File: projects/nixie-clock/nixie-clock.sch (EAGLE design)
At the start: 75 parts, among them J1 POWER JACK, T1 BC337, T2 BC337, T3 BC337, U1 DC-DC Converter, U2 K155ID1, U3 Arduino Pro Mini, U4 Pollin DCF1, U5 REG1117

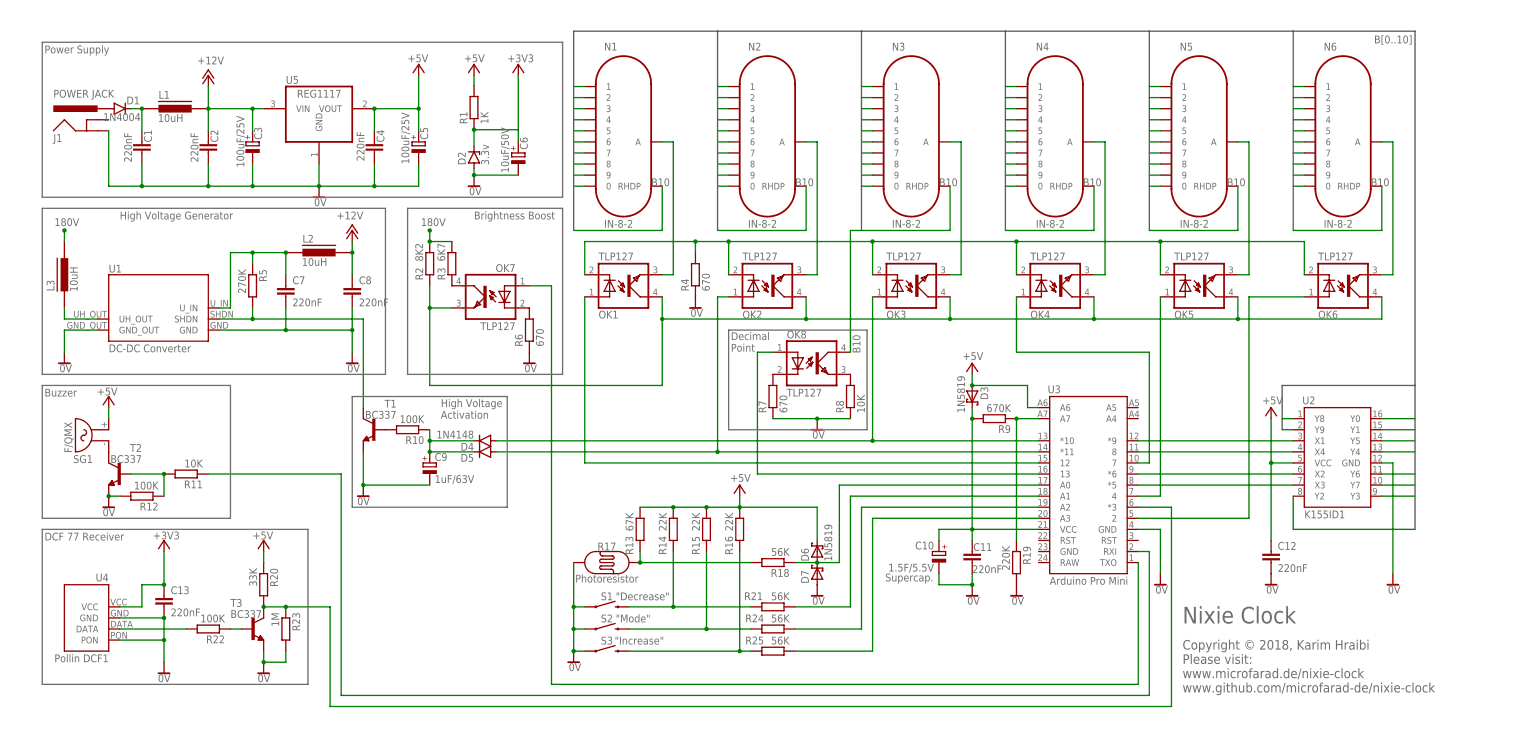
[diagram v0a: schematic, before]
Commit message: Update schematic
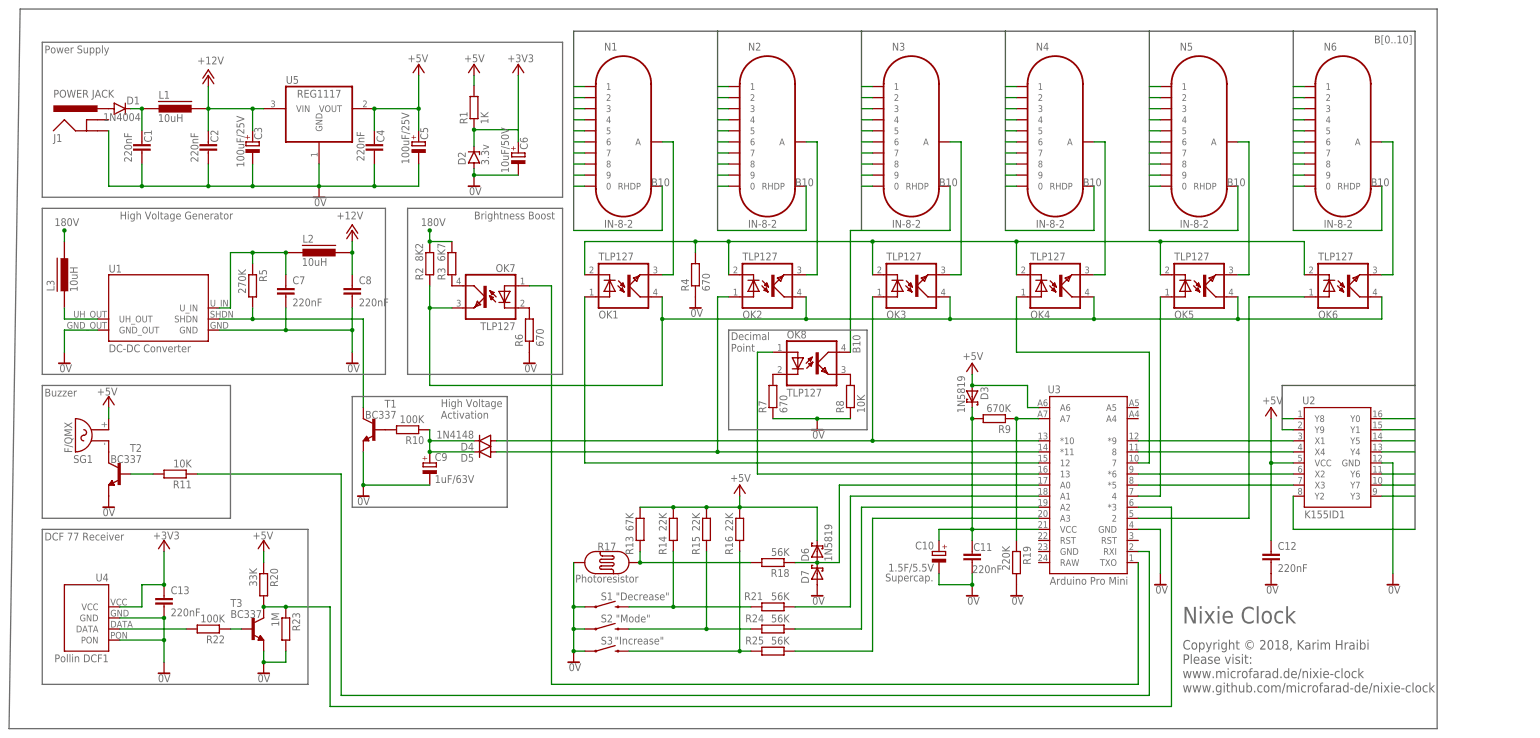
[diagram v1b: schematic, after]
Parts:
- removed R12: 100K, rcl:R-EU_0207/7
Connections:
- net 0V: no longer R12.2
- net N$28: no longer R12.1
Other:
- moved on the sheet: R11
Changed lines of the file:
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@@
 <part name="D7" library="diode" library_urn="urn:adsk.eagle:library:210" deviceset="1N581*" device="" package3d_urn="urn:adsk.eagle:package:43421/1" technology="9-B"/>
 <part name="SUPPLY13" library="supply2" library_urn="urn:adsk.eagle:library:372" deviceset="0V" device=""/>
-<part name="R12" library="rcl" library_urn="urn:adsk.eagle:library:334" deviceset="R-EU_" device="0207/7" package3d_urn="urn:adsk.eagle:package:23493/2" value="100K"/>
 </parts>
 <sheets>
@@
 www.microfarad.de/nixie-clock
 www.github.com/microfarad-de/nixie-clock</text>
+<wire x1="-180.34" y1="96.52" x2="144.78" y2="96.52" width="0.1524" layer="95"/>
+<wire x1="144.78" y1="96.52" x2="144.78" y2="-68.58" width="0.1524" layer="95"/>
+<wire x1="144.78" y1="-68.58" x2="-182.88" y2="-68.58" width="0.1524" layer="95"/>
+<wire x1="-182.88" y1="-68.58" x2="-180.34" y2="96.52" width="0.1524" layer="95"/>
 </plain>
 <instances>
@@
 <attribute name="VALUE" x="-152.4" y="-7.62" size="1.778" layer="96" rot="MR0"/>
 </instance>
-<instance part="R11" gate="G$1" x="-142.24" y="-10.16" smashed="yes" rot="R180">
-<attribute name="NAME" x="-138.43" y="-11.6586" size="1.778" layer="95" rot="R180"/>
-<attribute name="VALUE" x="-138.43" y="-6.858" size="1.778" layer="96" rot="R180"/>
+<instance part="R11" gate="G$1" x="-144.78" y="-10.16" smashed="yes" rot="R180">
+<attribute name="NAME" x="-140.97" y="-11.6586" size="1.778" layer="95" rot="R180"/>
+<attribute name="VALUE" x="-140.97" y="-6.858" size="1.778" layer="96" rot="R180"/>
 </instance>
 <instance part="SUPPLY9" gate="0V" x="-160.02" y="-17.78" smashed="yes" rot="MR0">
@@
 <instance part="SUPPLY13" gate="0V" x="2.54" y="-38.1" smashed="yes">
 <attribute name="VALUE" x="1.397" y="-40.132" size="1.778" layer="96"/>
-</instance>
-<instance part="R12" gate="G$1" x="-152.4" y="-15.24" smashed="yes" rot="R180">
-<attribute name="NAME" x="-148.59" y="-16.7386" size="1.778" layer="95" rot="R180"/>
-<attribute name="VALUE" x="-148.59" y="-11.938" size="1.778" layer="96" rot="R180"/>
 </instance>
 </instances>
@@
 <pinref part="T2" gate="G$1" pin="E"/>
 <pinref part="SUPPLY9" gate="0V" pin="0V"/>
-<pinref part="R12" gate="G$1" pin="2"/>
-<wire x1="-157.48" y1="-15.24" x2="-160.02" y2="-15.24" width="0.1524" layer="91"/>
-<junction x="-160.02" y="-15.24"/>
 </segment>
 <segment>
@@
 <segment>
 <pinref part="R11" gate="G$1" pin="1"/>
-<wire x1="-137.16" y1="-10.16" x2="-106.68" y2="-10.16" width="0.1524" layer="91"/>
+<wire x1="-139.7" y1="-10.16" x2="-106.68" y2="-10.16" width="0.1524" layer="91"/>
 <wire x1="-106.68" y1="-10.16" x2="-106.68" y2="-60.96" width="0.1524" layer="91"/>
 <wire x1="-106.68" y1="-60.96" x2="78.74" y2="-60.96" width="0.1524" layer="91"/>
@@
 <pinref part="R11" gate="G$1" pin="2"/>
 <pinref part="T2" gate="G$1" pin="B"/>
-<wire x1="-147.32" y1="-10.16" x2="-154.94" y2="-10.16" width="0.1524" layer="91"/>
-<wire x1="-147.32" y1="-15.24" x2="-147.32" y2="-10.16" width="0.1524" layer="91"/>
-<junction x="-147.32" y="-10.16"/>
-<pinref part="R12" gate="G$1" pin="1"/>
-</segment>
-</net>
+<wire x1="-149.86" y1="-10.16" x2="-154.94" y2="-10.16" width="0.1524" layer="91"/>
+</segment>
+</net>
